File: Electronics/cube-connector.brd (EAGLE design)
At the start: 15 x 15 mm, 4 parts

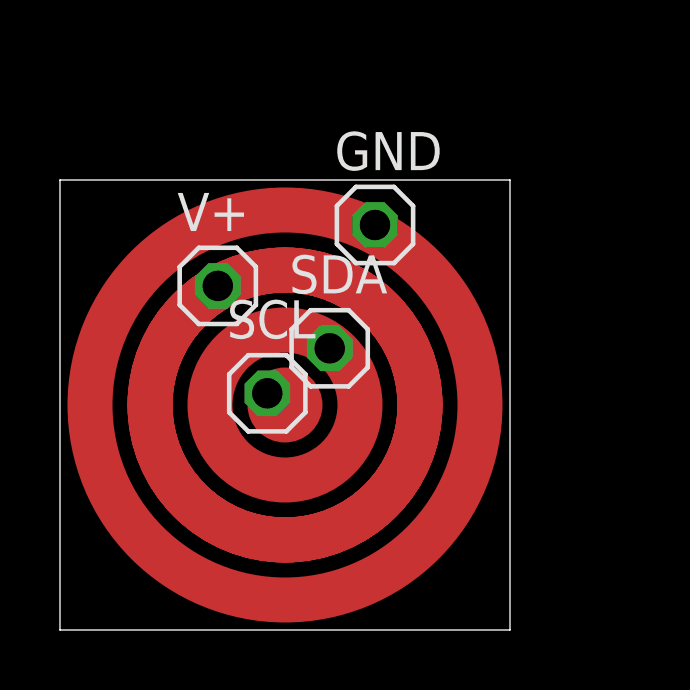
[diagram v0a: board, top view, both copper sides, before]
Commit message: File organising...
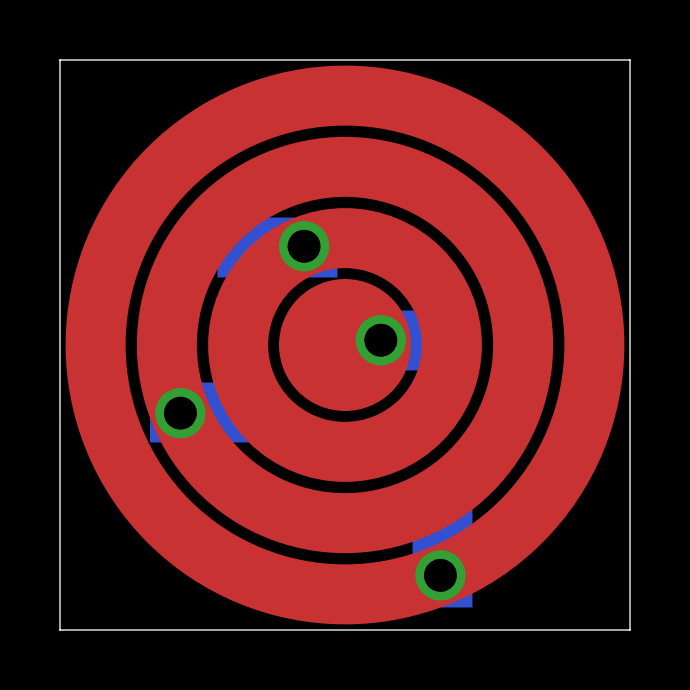
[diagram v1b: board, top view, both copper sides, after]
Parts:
- removed GND, SCL, SDA, V+: (no value), pinhead:1X01
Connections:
- removed net GND: GND.1
- removed net SCL: SCL.1
- removed net SDA: SDA.1
- removed net V+: V+.1
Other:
- board size 15 x 15 mm -> 19 x 19 mm
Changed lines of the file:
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@@
 <setting verticaltext="up"/>
 </settings>
-<grid distance="0.5" unitdist="mm" unit="mm" style="lines" multiple="1" display="no" altdistance="0.025" altunitdist="inch" altunit="mm"/>
+<grid distance="0.25" unitdist="mm" unit="mm" style="lines" multiple="1" display="no" altdistance="0.025" altunitdist="inch" altunit="mm"/>
 <layers>
 <layer number="1" name="Top" color="4" fill="1" visible="yes" active="yes"/>
@@
 <layer number="19" name="Unrouted" color="6" fill="1" visible="yes" active="yes"/>
 <layer number="20" name="Dimension" color="15" fill="1" visible="yes" active="yes"/>
-<layer number="21" name="tPlace" color="7" fill="1" visible="no" active="yes"/>
-<layer number="22" name="bPlace" color="7" fill="1" visible="no" active="yes"/>
+<layer number="21" name="tPlace" color="7" fill="1" visible="yes" active="yes"/>
+<layer number="22" name="bPlace" color="7" fill="1" visible="yes" active="yes"/>
 <layer number="23" name="tOrigins" color="15" fill="1" visible="yes" active="yes"/>
 <layer number="24" name="bOrigins" color="15" fill="1" visible="yes" active="yes"/>
@@
 <board>
 <plain>
-<wire x1="0" y1="0" x2="15" y2="0" width="0" layer="20"/>
-<wire x1="15" y1="0" x2="15" y2="15" width="0" layer="20"/>
-<wire x1="15" y1="15" x2="0" y2="15" width="0" layer="20"/>
-<wire x1="0" y1="15" x2="0" y2="0" width="0" layer="20"/>
-<circle x="7.5" y="7.5" radius="4.5" width="1.5" layer="1"/>
-<circle x="7.5" y="7.5" radius="1.25" width="0" layer="1"/>
-<circle x="7.5" y="7.5" radius="6.5" width="1.5" layer="1"/>
-<circle x="7.5" y="7.5" radius="2.5" width="1.5" layer="1"/>
-<circle x="7.5" y="7.5" radius="4.5" width="1.5" layer="1"/>
+<wire x1="0" y1="0" x2="19" y2="0" width="0" layer="20"/>
+<wire x1="19" y1="0" x2="19" y2="19" width="0" layer="20"/>
+<wire x1="19" y1="19" x2="0" y2="19" width="0" layer="20"/>
+<wire x1="0" y1="19" x2="0" y2="0" width="0" layer="20"/>
+<circle x="9.5" y="9.5" radius="2.2" width="0" layer="1"/>
+<circle x="9.5" y="9.5" radius="3.563" width="2" layer="1"/>
+<circle x="9.5" y="9.5" radius="5.938" width="2" layer="1"/>
+<circle x="9.5" y="9.5" radius="8.313" width="2" layer="1"/>
+<rectangle x1="3" y1="6.25" x2="7" y2="8.25" layer="16"/>
+<rectangle x1="5.25" y1="11.75" x2="9.25" y2="13.75" layer="16"/>
+<rectangle x1="9.75" y1="8.65" x2="13.75" y2="10.65" layer="16"/>
+<rectangle x1="10.75" y1="1.75" x2="14.75" y2="3.75" layer="16" rot="R270"/>
 </plain>
 <attributes>
@@
 </autorouter>
 <elements>
-<element name="GND" library="pinhead" package="1X01" value="" x="10.5" y="13.5"/>
-<element name="SCL" library="pinhead" package="1X01" value="" x="6.91" y="7.89"/>
-<element name="SDA" library="pinhead" package="1X01" value="" x="8.99" y="9.39"/>
-<element name="V+" library="pinhead" package="1X01" value="" x="5.26" y="11.47"/>
 </elements>
 <signals>
+<signal name="GND">
+<via x="12.681" y="1.82" extent="1-16" drill="1.1" diameter="1.6764"/>
+</signal>
 <signal name="V+">
-<contactref element="V+" pad="1"/>
-</signal>
-<signal name="GND">
-<contactref element="GND" pad="1"/>
+<via x="10.694" y="9.658" extent="1-16" drill="1.1" diameter="1.6764"/>
 </signal>
 <signal name="SDA">
-<contactref element="SDA" pad="1"/>
+<via x="8.137" y="12.791" extent="1-16" drill="1.1" diameter="1.6764"/>
 </signal>
 <signal name="SCL">
-<contactref element="SCL" pad="1"/>
+<via x="4.014" y="7.228" extent="1-16" drill="1.1" diameter="1.6764"/>
 </signal>
 </signals>
